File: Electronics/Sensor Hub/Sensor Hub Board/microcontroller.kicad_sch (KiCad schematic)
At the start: 57 parts, among them IC301 TJA1057GT/3, IC302 STM32H723ZGT6, J301 TC2030, J302 Pluggable_Terminal_01x03, J303 TYPE-C-31-M-12, J417 JST_SH_1mm_1x4, SW301 SW_DIP_x02, U301 USBLC6-4SC6-ES, U302 USBLC6-4SC6-ES, X301 25MHz_Clock, X302 32.768kHz_Clock

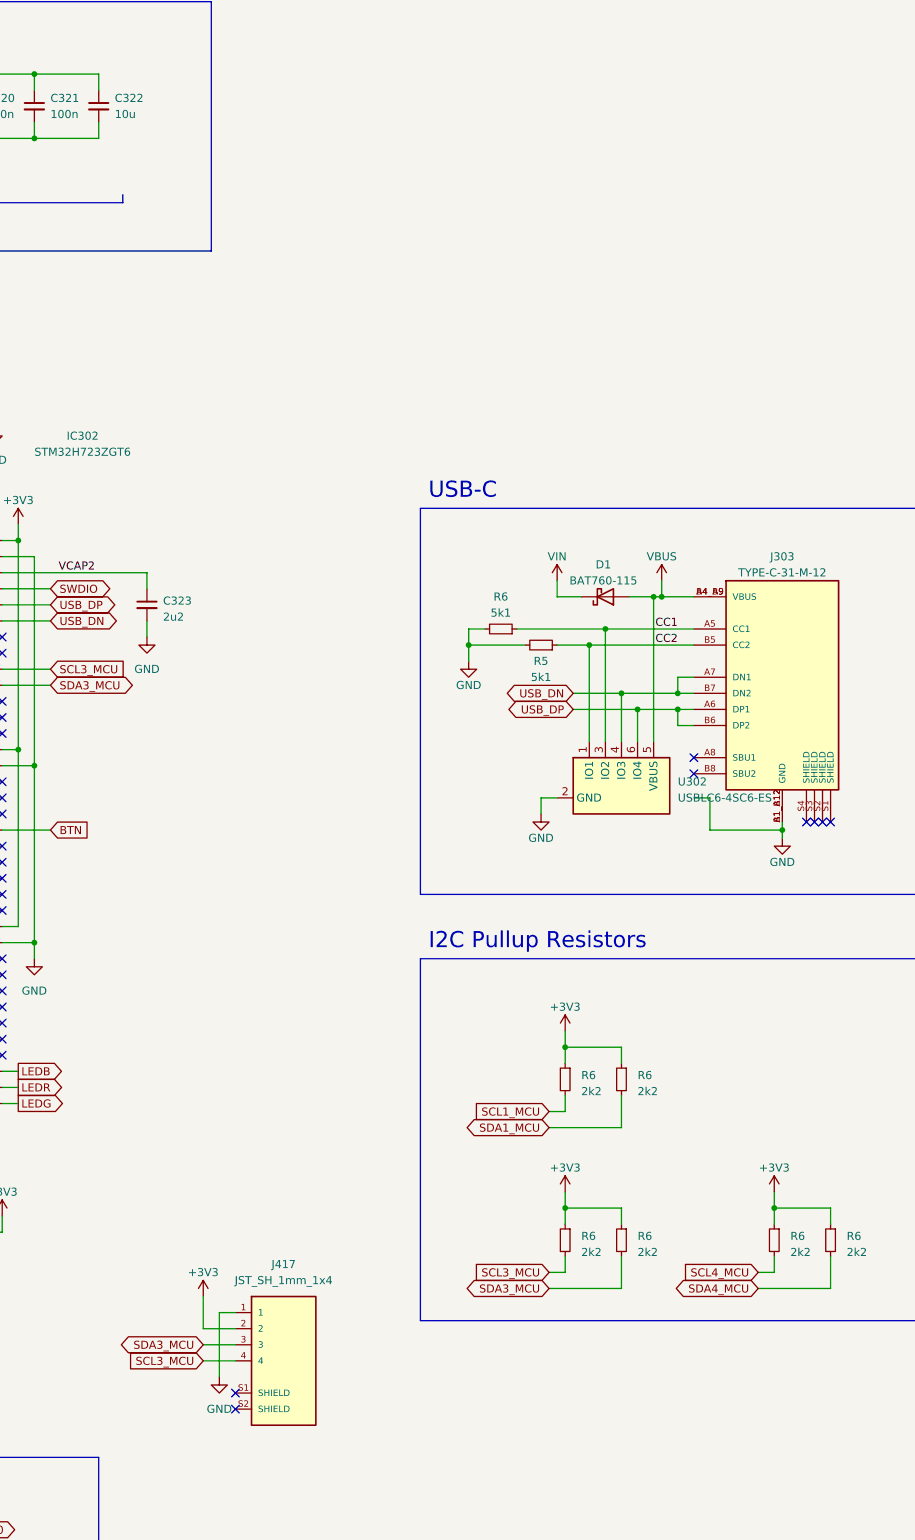
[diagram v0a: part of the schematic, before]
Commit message: All boards done
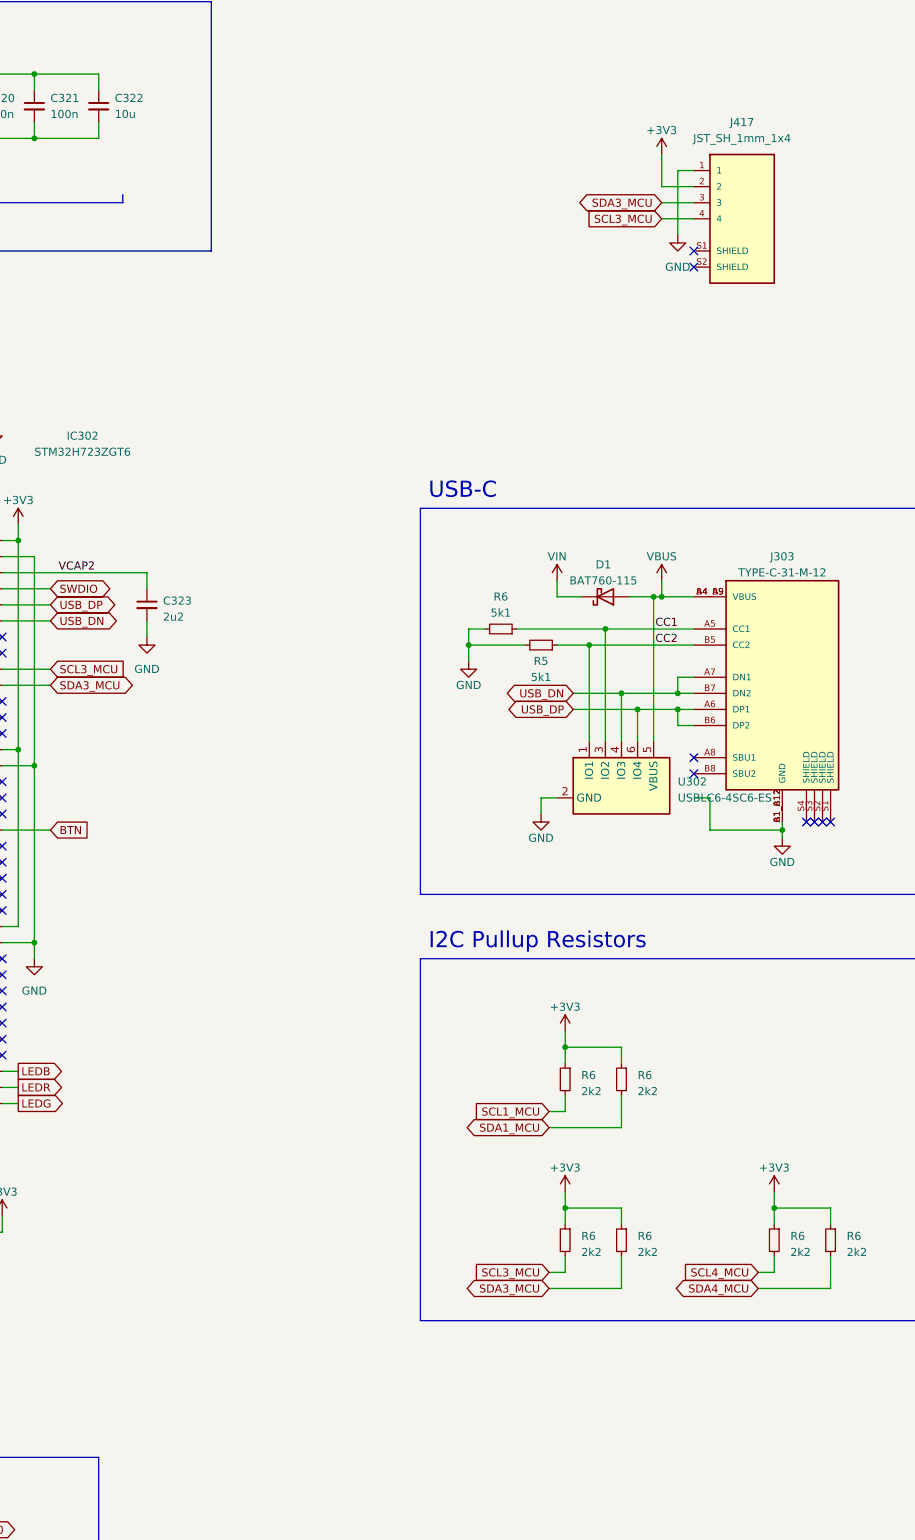
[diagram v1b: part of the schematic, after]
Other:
- moved on the sheet: J417
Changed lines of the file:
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@@
   (no_connect (at 36.83 210.82))
   (no_connect (at 245.11 143.51))
-  (no_connect (at 281.94 240.03))
+  (no_connect (at 354.33 59.69))
   (no_connect (at 245.11 133.35))
   (no_connect (at 245.11 176.53))
@@
   (no_connect (at 245.11 181.61))
   (no_connect (at 374.65 149.86))
-  (no_connect (at 281.94 242.57))
+  (no_connect (at 354.33 62.23))
   (no_connect (at 204.47 212.09))
   (no_connect (at 245.11 153.67))
@@
     (stroke (width 0) (type default))
   )
-  (wire (pts (xy 276.86 234.95) (xy 281.94 234.95))
+  (wire (pts (xy 349.25 54.61) (xy 354.33 54.61))
     (stroke (width 0) (type default))
   )
@@
     (stroke (width 0) (type default))
   )
-  (wire (pts (xy 279.4 227.33) (xy 279.4 237.49))
+  (wire (pts (xy 351.79 46.99) (xy 351.79 57.15))
     (stroke (width 0) (type default))
   )
@@
     (stroke (width 0) (type default))
   )
-  (wire (pts (xy 276.86 224.79) (xy 276.86 229.87))
+  (wire (pts (xy 349.25 44.45) (xy 349.25 49.53))
     (stroke (width 0) (type default))
   )
@@
     (stroke (width 0) (type default))
   )
-  (wire (pts (xy 281.94 227.33) (xy 279.4 227.33))
+  (wire (pts (xy 354.33 46.99) (xy 351.79 46.99))
     (stroke (width 0) (type default))
   )
@@
     (stroke (width 0) (type default))
   )
-  (wire (pts (xy 276.86 229.87) (xy 281.94 229.87))
+  (wire (pts (xy 349.25 49.53) (xy 354.33 49.53))
     (stroke (width 0) (type default))
   )
@@
     (stroke (width 0) (type default))
   )
-  (wire (pts (xy 276.86 232.41) (xy 281.94 232.41))
+  (wire (pts (xy 349.25 52.07) (xy 354.33 52.07))
     (stroke (width 0) (type default))
   )
@@
     )
   )
-  (global_label "SCL3_MCU" (shape input) (at 276.86 234.95 180) (fields_autoplaced)
+  (global_label "SCL3_MCU" (shape input) (at 349.25 54.61 180) (fields_autoplaced)
     (effects (font (size 1.27 1.27)) (justify right))
-    (property "Intersheetrefs" "${INTERSHEET_REFS}" (at 264.2176 234.95 0)
+    (property "Intersheetrefs" "${INTERSHEET_REFS}" (at 336.6076 54.61 0)
       (effects (font (size 1.27 1.27)) (justify right) hide)
     )
@@
     )
   )
-  (global_label "SDA3_MCU" (shape bidirectional) (at 276.86 232.41 180) (fields_autoplaced)
+  (global_label "SDA3_MCU" (shape bidirectional) (at 349.25 52.07 180) (fields_autoplaced)
     (effects (font (size 1.27 1.27)) (justify right))
-    (property "Intersheetrefs" "${INTERSHEET_REFS}" (at 263.0458 232.41 0)
+    (property "Intersheetrefs" "${INTERSHEET_REFS}" (at 335.4358 52.07 0)
       (effects (font (size 1.27 1.27)) (justify right) hide)
     )
@@
     )
   )
-  (symbol (lib_id "power:GND") (at 279.4 237.49 0) (unit 1)
+  (symbol (lib_id "power:GND") (at 351.79 57.15 0) (unit 1)
     (in_bom yes) (on_board yes) (dnp no) (fields_autoplaced)
-    (property "Reference" "#PWR0441" (at 279.4 243.84 0)
+    (property "Reference" "#PWR0441" (at 351.79 63.5 0)
       (effects (font (size 1.27 1.27)) hide)
     )
-    (property "Value" "GND" (at 279.4 242.57 0)
+    (property "Value" "GND" (at 351.79 62.23 0)
       (effects (font (size 1.27 1.27)))
     )
-    (property "Footprint" "" (at 279.4 237.49 0)
+    (property "Footprint" "" (at 351.79 57.15 0)
       (effects (font (size 1.27 1.27)) hide)
     )
-    (property "Datasheet" "" (at 279.4 237.49 0)
+    (property "Datasheet" "" (at 351.79 57.15 0)
       (effects (font (size 1.27 1.27)) hide)
     )
@@
     )
   )
-  (symbol (lib_id "power:+3V3") (at 276.86 224.79 0) (unit 1)
+  (symbol (lib_id "power:+3V3") (at 349.25 44.45 0) (unit 1)
     (in_bom yes) (on_board yes) (dnp no) (fields_autoplaced)
-    (property "Reference" "#PWR0442" (at 276.86 228.6 0)
+    (property "Reference" "#PWR0442" (at 349.25 48.26 0)
       (effects (font (size 1.27 1.27)) hide)
     )
-    (property "Value" "+3V3" (at 276.86 220.98 0)
+    (property "Value" "+3V3" (at 349.25 40.64 0)
       (effects (font (size 1.27 1.27)))
     )
-    (property "Footprint" "" (at 276.86 224.79 0)
+    (property "Footprint" "" (at 349.25 44.45 0)
       (effects (font (size 1.27 1.27)) hide)
     )
-    (property "Datasheet" "" (at 276.86 224.79 0)
+    (property "Datasheet" "" (at 349.25 44.45 0)
       (effects (font (size 1.27 1.27)) hide)
     )
@@
     )
   )
-  (symbol (lib_id "MSL_Symbols:JST_SH_1mm_1x4") (at 289.56 232.41 0) (unit 1)
+  (symbol (lib_id "MSL_Symbols:JST_SH_1mm_1x4") (at 361.95 52.07 0) (unit 1)
     (in_bom yes) (on_board yes) (dnp no)
-    (property "Reference" "J417" (at 289.56 219.71 0)
+    (property "Reference" "J417" (at 361.95 39.37 0)
       (effects (font (size 1.27 1.27)))
     )
-    (property "Value" "JST_SH_1mm_1x4" (at 289.56 222.25 0)
+    (property "Value" "JST_SH_1mm_1x4" (at 361.95 41.91 0)
       (effects (font (size 1.27 1.27)))
     )
-    (property "Footprint" "MSL Footprints:JST_SH_1mm_1x4" (at 289.56 232.41 0)
+    (property "Footprint" "MSL Footprints:JST_SH_1mm_1x4" (at 361.95 52.07 0)
       (effects (font (size 1.27 1.27)) (justify bottom) hide)
     )
-    (property "Datasheet" "" (at 289.56 232.41 0)
+    (property "Datasheet" "" (at 361.95 52.07 0)
       (effects (font (size 1.27 1.27)) hide)
     )
-    (property "MANUFACTURER" "JST" (at 289.56 232.41 0)
+    (property "MANUFACTURER" "JST" (at 361.95 52.07 0)
       (effects (font (size 1.27 1.27)) (justify bottom) hide)
     )
-    (property "STANDARD" "Manufacturer recommendations" (at 289.56 232.41 0)
+    (property "STANDARD" "Manufacturer recommendations" (at 361.95 52.07 0)
       (effects (font (size 1.27 1.27)) (justify bottom) hide)
     )
